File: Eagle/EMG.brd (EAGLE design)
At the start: 141.9 x 86.3 mm, 45 parts, among them IC1 AD623N, IC2 OPA344P, IC3 OPA344P, IC4 OPA344P, IC5 OPA344P, IC6 OPA344P, IC7 OPA344P, IC9 MAX339CPE

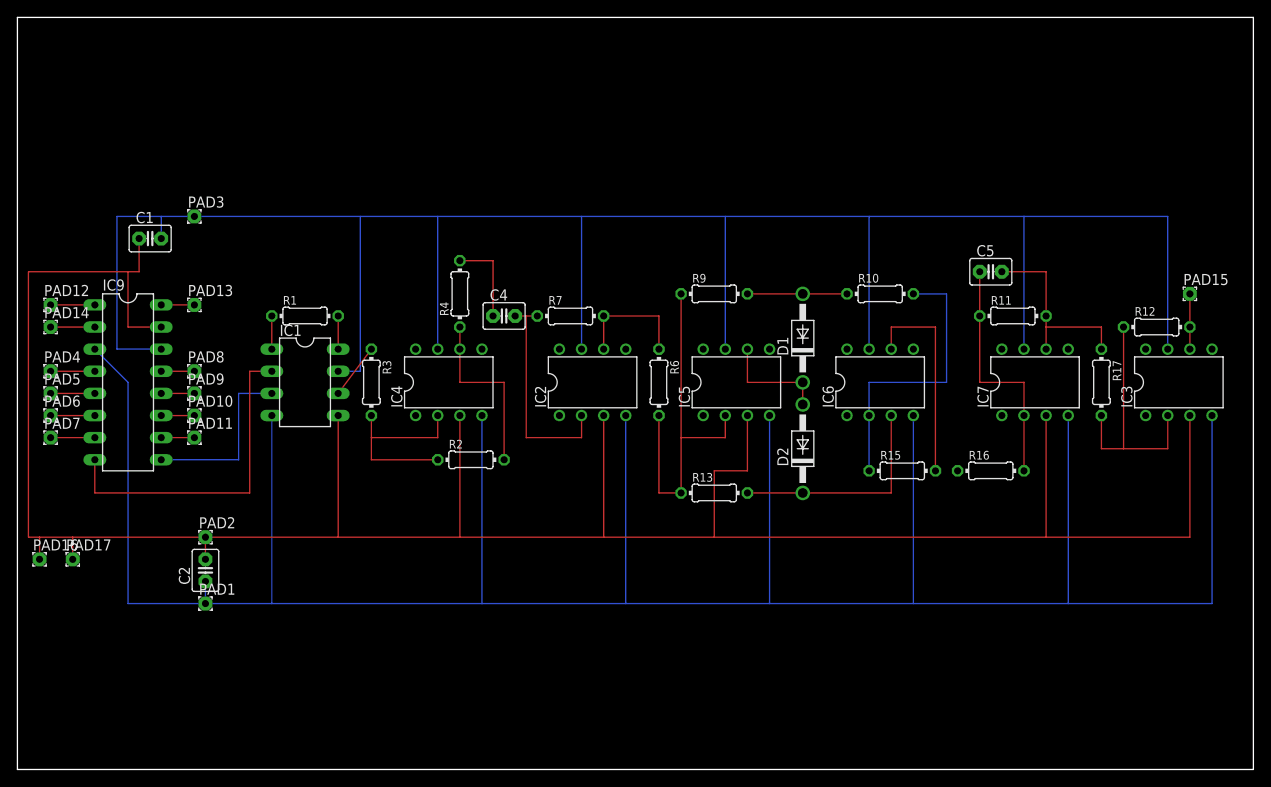
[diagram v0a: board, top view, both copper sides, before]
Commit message: Compressed brd
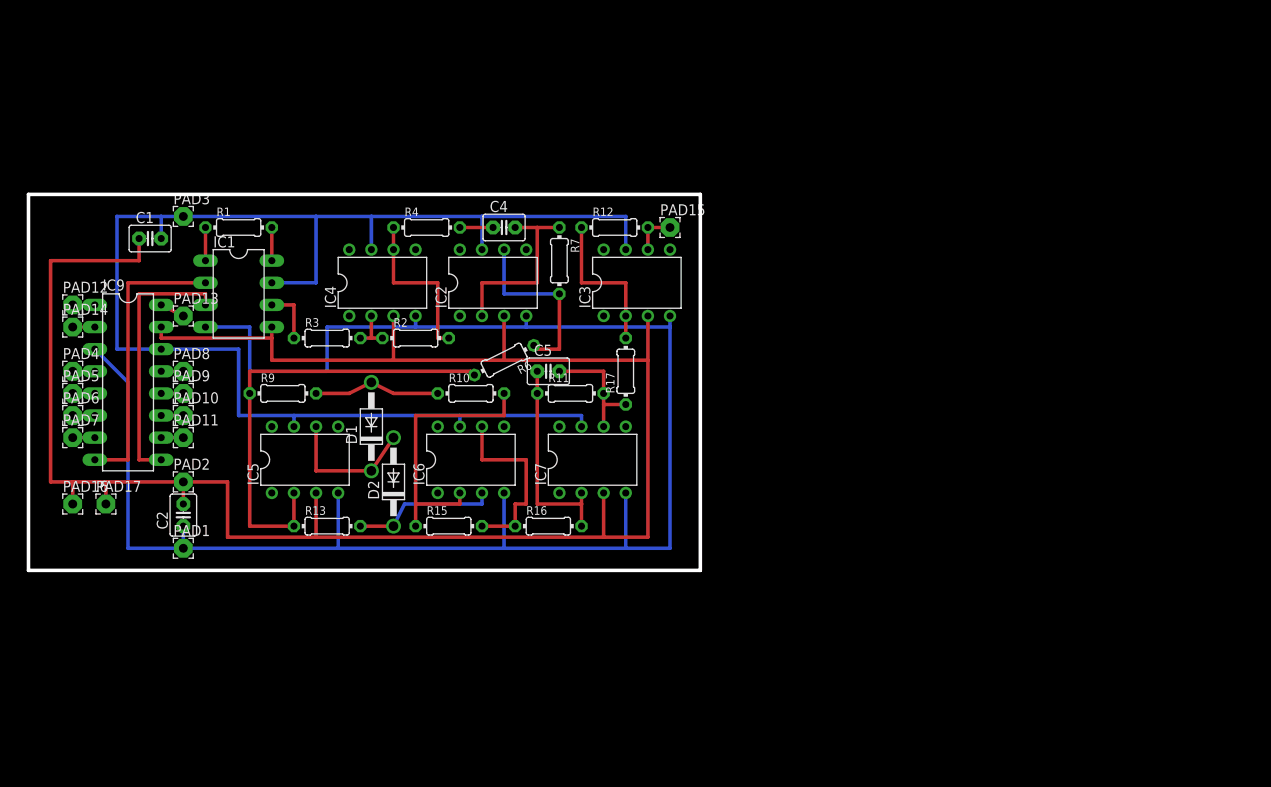
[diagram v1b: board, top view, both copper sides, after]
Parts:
- PAD1, PAD10, PAD11, PAD12, PAD13, PAD14, PAD15, PAD16, PAD17, PAD2, PAD3, PAD4, PAD5, PAD6, PAD7, PAD8, PAD9: device wirepad:1,6/0,8 -> wirepad:2,15/1,0
- moved R12 63.3 mm to (68.6, 55.9)
- moved IC3 63.3 mm to (71.1, 49.5)
- moved PAD15 60.2 mm to (74.9, 55.9)
- moved R17 54.6 mm to (69.8, 39.4), turned to 90 degrees
- moved R15 52.5 mm to (49.5, 21.6)
- moved C5 52.1 mm to (61.0, 39.4)
- moved IC7 51.6 mm to (66.0, 29.2)
- moved R11 51.6 mm to (63.5, 36.8)
- moved R16 51.2 mm to (61.0, 21.6)
- moved R9 50.8 mm to (30.5, 36.8)
- moved D1 50.6 mm to (40.6, 33.0)
- moved IC5 50.3 mm to (33.0, 29.2)
- moved R10 48.4 mm to (52.1, 36.8)
- moved IC6 47.8 mm to (52.1, 29.2)
- moved D2 47.1 mm to (43.2, 26.7)
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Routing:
- net -9V: track 308.9 -> 201.0 mm
- net +9V: track 255.3 -> 165.1 mm
- net GND: track 285.8 -> 227.3 mm
- net N$4: track 22.9 -> 5.08 mm
- net N$15: track 29.2 -> 17.8 mm
- net N$9: track 41.9 -> 52.6 mm
- net N$21: track 20.3 -> 30.5 mm
- net N$14: track 22.9 -> 14.0 mm
- net N$17: track 25.4 -> 16.8 mm
- net N$11: track 14.0 -> 20.9 mm
- net N$7: track 10.2 -> 3.81 mm
- net N$20: track 38.1 -> 33.0 mm
- net N$13: track 27.9 -> 24.1 mm
- net N$8: track 25.4 -> 21.6 mm
- net N$18: track 12.7 -> 16.0 mm
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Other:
- board size 141.9 x 86.3 mm -> 77.1 x 43.2 mm
